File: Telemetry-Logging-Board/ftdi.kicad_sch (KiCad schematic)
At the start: 2 parts, among them P1 USB_C_Plug_USB2.0, U8 FT230XQ

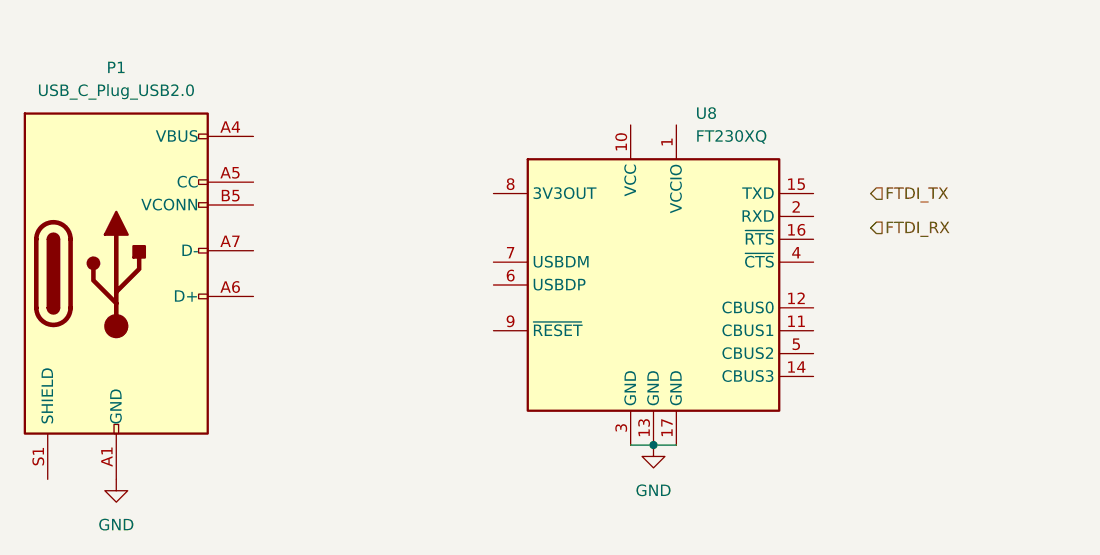
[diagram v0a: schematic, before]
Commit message: FTDI
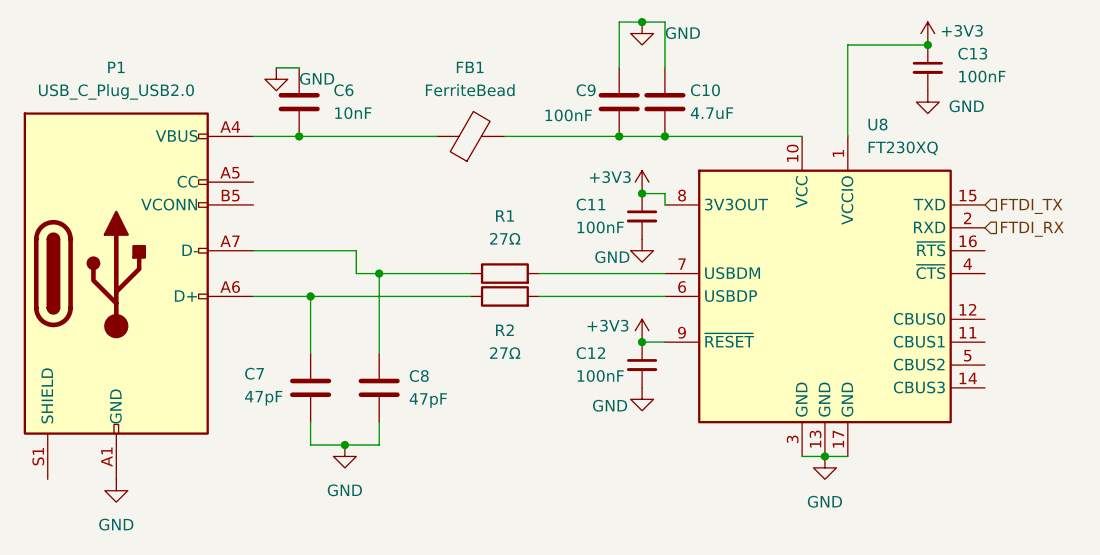
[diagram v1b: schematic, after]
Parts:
- added C10: 4.7uF, symbol Device:C
- added C11, C12, C13: 100nF, symbol Device:C_Small
- added C6: 10nF, symbol Device:C
- added C7, C8: 47pF, symbol Device:C
- added C9: 100nF, symbol Device:C
- added FB1: FerriteBead, symbol Device:FerriteBead
- added R1, R2: 27Ω, symbol Device:R
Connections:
- net FTDI_RX: now also U8.2 (RXD)
- net FTDI_TX: now also U8.15 (TXD)
- net GND: now also C10.1, C11.2, C12.2, C13.2, C6.1, C7.2, C8.2, C9.1
- net +3V3: now reaches U8.1 (VCCIO)
- net +3V3: now also U8.8 (3V3OUT), U8.9 (~{RESET}), C11.1, C12.1, C13.1
- net at U8.10 (VCC): now also C10.2, C9.2, FB1.2
- net at U8.6 (USBDP): now also R2.2
- net at U8.7 (USBDM): now also R1.2
- net at P1.A4 (VBUS), P1.A9 (VBUS), P1.B4 (VBUS)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: now also C6.2, FB1.1
- net at P1.A6 (D+): now also C7.1, R2.1
- net at P1.A7 (D-): now also C8.1, R1.1
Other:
- moved on the sheet: U8
